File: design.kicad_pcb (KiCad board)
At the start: 2 copper layers, 81.5 x 51 mm, 26 parts, among them J1 490107670412, J2 TYPE-C-31-M-12, J4 Conn_02x02_Counter_Clockwise, SW3 EN, U1 AP2112K-3.3, U2 TCK107AF,LF, U3 CH340C, U4 TS3USB30RSWR

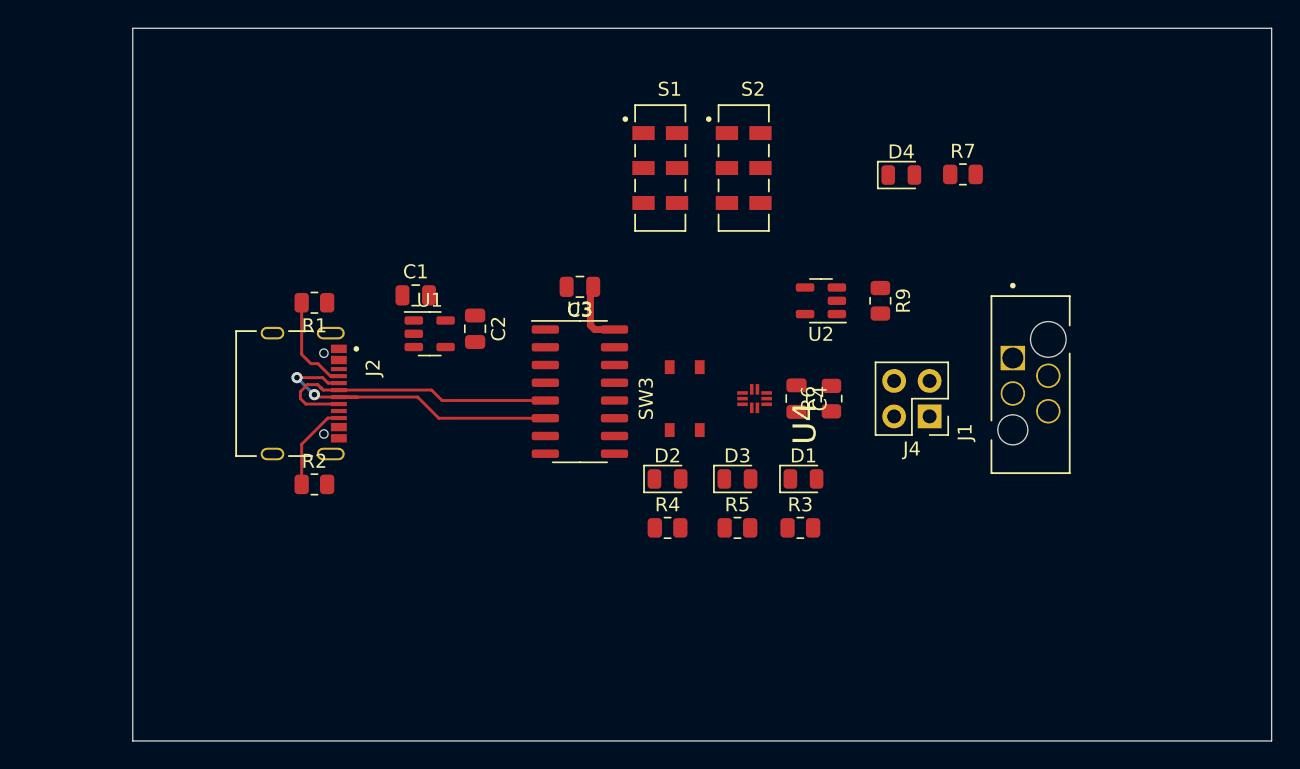
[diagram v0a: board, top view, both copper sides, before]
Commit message: update
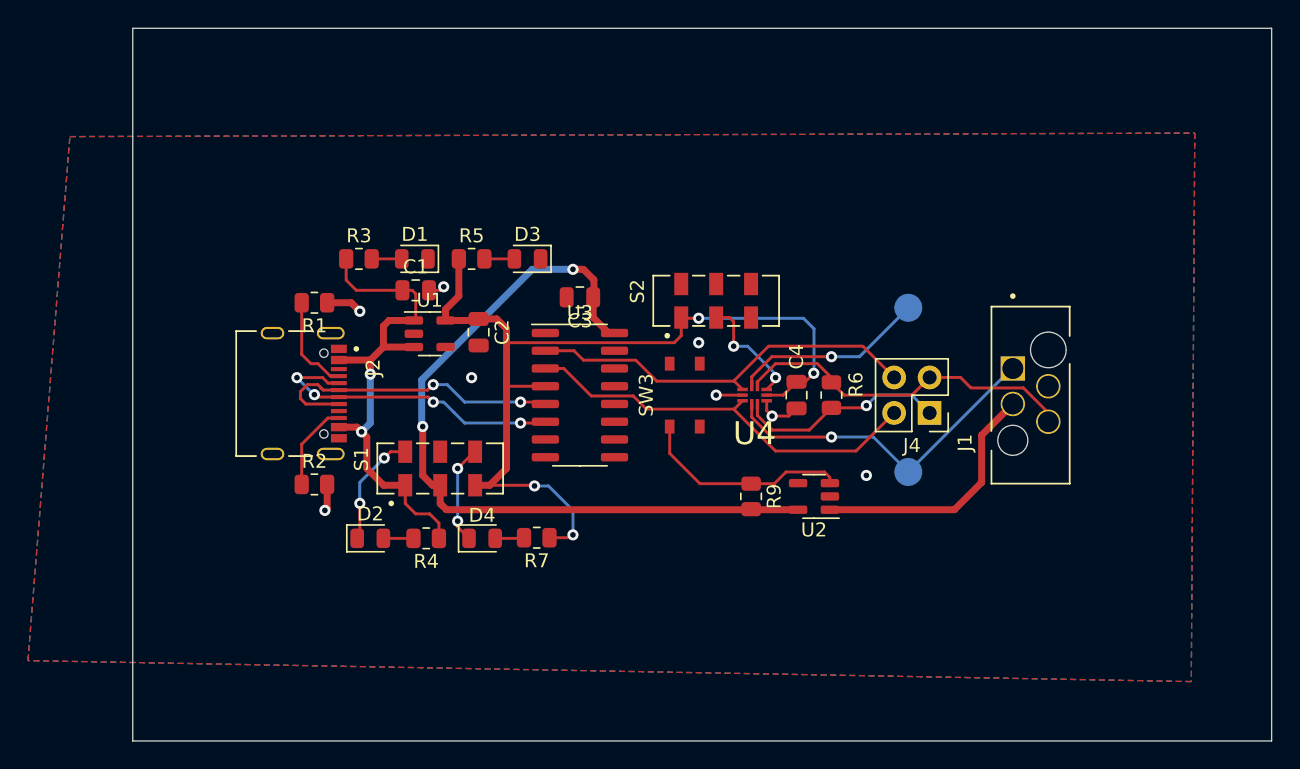
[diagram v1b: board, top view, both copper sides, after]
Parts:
- added REF**: TestPoint_Pad_D2.0mm, TestPoint:TestPoint_Pad_D2.0mm, B.Cu at (164.5, 88.5)
- added REF**: TestPoint_Pad_D2.0mm, TestPoint:TestPoint_Pad_D2.0mm, B.Cu at (164.5, 100.2)
- moved R7 40.1 mm to (137.9, 105.0), turned to 180 degrees
- moved D4 39.7 mm to (134.0, 105.0)
- moved R3 37.0 mm to (125.2, 85.0)
- moved D1 32.0 mm to (129.2, 85.0), turned to 180 degrees
- moved R5 27.1 mm to (133.2, 85.0)
- moved S1 26.7 mm to (131.0, 100.0), turned to 90 degrees
- moved D3 21.8 mm to (137.2, 85.0), turned to 180 degrees
- moved D2 21.7 mm to (126.0, 105.0)
- moved R4 17.3 mm to (130.0, 105.0), turned to 180 degrees
- moved R9 16.8 mm to (153.2, 102.0)
- moved U2 14.0 mm to (157.8, 102.0)
- moved S2 9.70 mm to (150.8, 88.0), turned to 90 degrees
- moved C3 0.75 mm to (141.0, 87.8)
- moved J1 0.75 mm to (173.2, 94.8)
- moved C1 0.36 mm to (129.2, 87.2)
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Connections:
- J1 pad 1: RX1 -> RX2
- J2 pad S1: Net-(J2-PadS1) -> unconnected-(J2-PadS1)
- J2 pad S2: Net-(J2-PadS1) -> unconnected-(J2-PadS1)
- J2 pad S3: Net-(J2-PadS1) -> unconnected-(J2-PadS1)
- J2 pad S4: Net-(J2-PadS1) -> unconnected-(J2-PadS1)
- J4 pad 1: TX1 -> RX1
- J4 pad 2: TX -> RX
- J4 pad 3: RX1 -> TX1
- J4 pad 4: RX -> TX
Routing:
- net +3V3: track 0.00 -> 67.4 mm, vias 0 -> 4
- net VDD: track 4.68 -> 56.1 mm, vias 0 -> 2
- net VBUS: track 0.00 -> 37.0 mm, vias 0 -> 2
- net RX: track 0.00 -> 29.4 mm
- net TX: track 0.00 -> 28.7 mm
- net TX1: track 0.00 -> 25.0 mm
- net RX2: track 0.00 -> 24.3 mm, vias 0 -> 1
- net VCC: track 0.00 -> 18.2 mm
- net Net-(R9-Pad1): track 0.00 -> 15.2 mm
- net RX1: track 0.00 -> 15.1 mm, vias 0 -> 1
- net TX2: track 0.00 -> 13.9 mm, vias 0 -> 1
- net GND: track 0.05 -> 10.8 mm, vias 0 -> 8
- net Switch: track 0.00 -> 8.31 mm, vias 0 -> 2
- net Net-(D2-Pad1): track 0.00 -> 8.24 mm, vias 0 -> 2
- net Net-(D4-Pad1): track 0.00 -> 7.08 mm, vias 0 -> 2
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- added copper zone on B.Cu, net GND
- added copper zone on F.Cu, net GND
